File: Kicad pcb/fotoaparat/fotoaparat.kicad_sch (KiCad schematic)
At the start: 71 parts, among them IC1 Lineární Regulátor, IC3 Lineární Regulátor Displaye, J1 USB Konektor, J2 SWD, J3 LCD konektor, J4 Baterie, J5 GSD090012SEU, J6 UART, J7 Kamera, J9 Conn_01x11_Socket, U1 STM32L496RETx, U2 MCP73833-FCI/UN, Y1 8mhz krystal

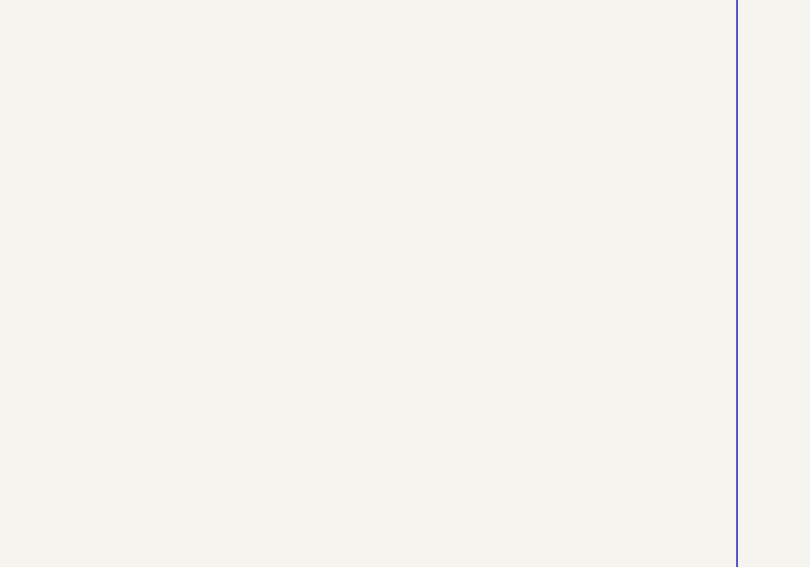
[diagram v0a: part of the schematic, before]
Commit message: Outline desky
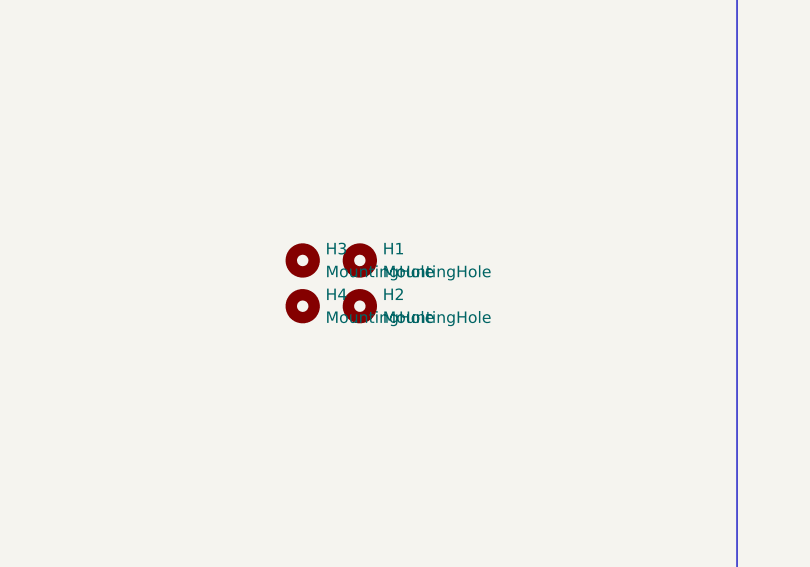
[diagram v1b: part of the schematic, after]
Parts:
- added H1, H2, H3, H4: MountingHole, MountingHole:MountingHole_3.2mm_M3, symbol Mechanical:MountingHole

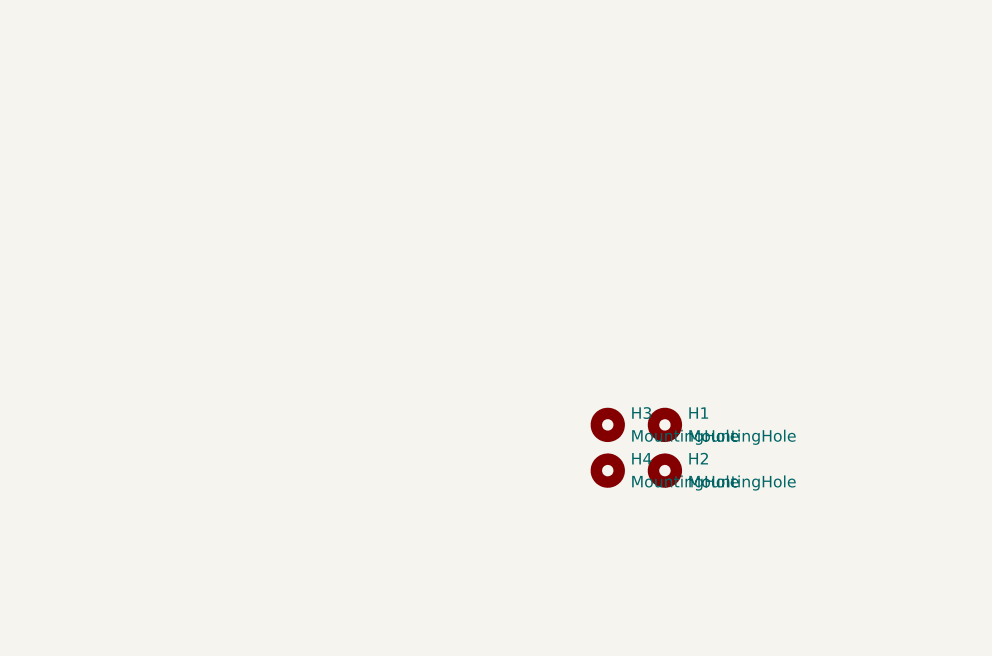
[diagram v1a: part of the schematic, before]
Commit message: První prototyp pcb
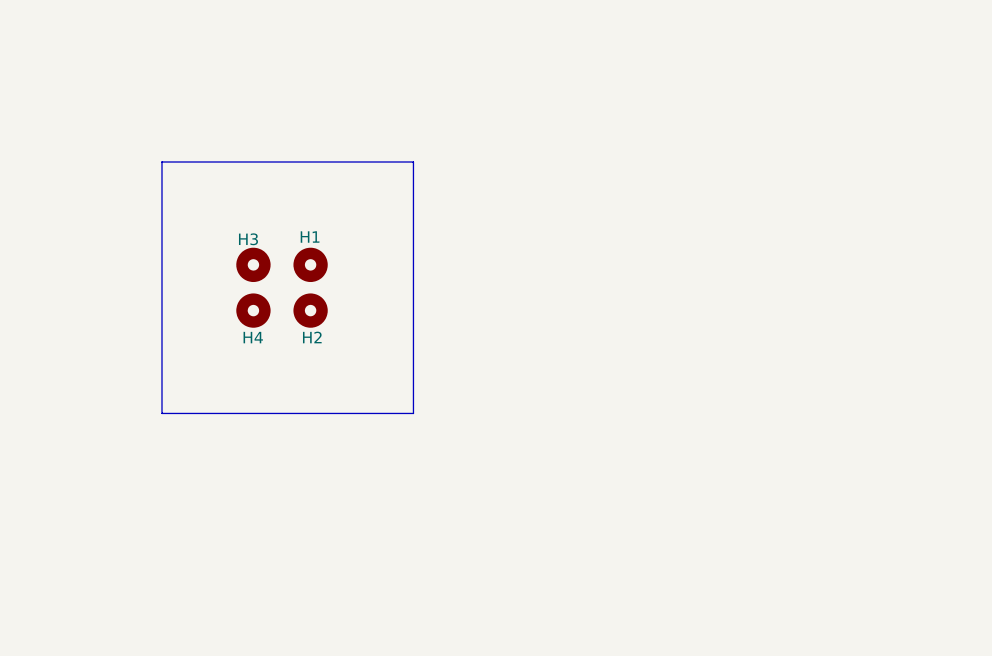
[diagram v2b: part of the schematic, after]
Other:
- moved on the sheet: H1, H2, H3, H4
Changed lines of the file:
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@@
 		(company "Vilem Maly")
 	)
+	(rectangle
+		(start -69.85 26.67)
+		(end -41.91 54.61)
+		(stroke
+			(width 0)
+			(type default)
+		)
+		(fill
+			(type none)
+		)
+	)
 	(text "Stm32 mikrokontrolér"
 		(exclude_from_sim no)
@@
 	(symbol
 		(lib_id "Mechanical:MountingHole")
-		(at -13.97 60.96 0)
+		(at -53.34 43.18 0)
 		(unit 1)
 		(exclude_from_sim no)
@@
 		(on_board yes)
 		(dnp no)
-		(fields_autoplaced yes)
 		(property "Reference" "H2"
-			(at -11.43 59.6899 0)
+			(at -54.356 46.228 0)
 			(effects
 				(font
@@
 		)
 		(property "Value" "MountingHole"
-			(at -11.43 62.2299 0)
+			(at -50.8 44.4499 0)
 			(effects
 				(font
@@
 				)
 				(justify left)
+				(hide yes)
 			)
 		)
 		(property "Footprint" "MountingHole:MountingHole_3.2mm_M3"
-			(at -13.97 60.96 0)
+			(at -53.34 43.18 0)
 			(effects
 				(font
@@
 		)
 		(property "Datasheet" "~"
-			(at -13.97 60.96 0)
+			(at -53.34 43.18 0)
 			(effects
 				(font
@@
 		)
 		(property "Description" "Mounting Hole without connection"
-			(at -13.97 60.96 0)
+			(at -53.34 43.18 0)
 			(effects
 				(font
@@
 	(symbol
 		(lib_id "Mechanical:MountingHole")
-		(at -20.32 60.96 0)
+		(at -59.69 43.18 0)
 		(unit 1)
 		(exclude_from_sim no)
@@
 		(on_board yes)
 		(dnp no)
-		(fields_autoplaced yes)
 		(property "Reference" "H4"
-			(at -17.78 59.6899 0)
+			(at -60.96 46.228 0)
 			(effects
 				(font
@@
 		)
 		(property "Value" "MountingHole"
-			(at -17.78 62.2299 0)
+			(at -57.15 44.4499 0)
 			(effects
 				(font
@@
 				)
 				(justify left)
+				(hide yes)
 			)
 		)
 		(property "Footprint" "MountingHole:MountingHole_3.2mm_M3"
-			(at -20.32 60.96 0)
+			(at -59.69 43.18 0)
 			(effects
 				(font
@@
 		)
 		(property "Datasheet" "~"
-			(at -20.32 60.96 0)
+			(at -59.69 43.18 0)
 			(effects
 				(font
@@
 		)
 		(property "Description" "Mounting Hole without connection"
-			(at -20.32 60.96 0)
+			(at -59.69 43.18 0)
 			(effects
 				(font
@@
 	(symbol
 		(lib_id "Mechanical:MountingHole")
-		(at -13.97 55.88 0)
+		(at -53.34 38.1 0)
 		(unit 1)
 		(exclude_from_sim no)
@@
 		(on_board yes)
 		(dnp no)
-		(fields_autoplaced yes)
 		(property "Reference" "H1"
-			(at -11.43 54.6099 0)
+			(at -54.61 35.052 0)
 			(effects
 				(font
@@
 		)
 		(property "Value" "MountingHole"
-			(at -11.43 57.1499 0)
+			(at -50.8 39.3699 0)
 			(effects
 				(font
@@
 				)
 				(justify left)
+				(hide yes)
 			)
 		)
 		(property "Footprint" "MountingHole:MountingHole_3.2mm_M3"
-			(at -13.97 55.88 0)
+			(at -53.34 38.1 0)
 			(effects
 				(font
@@
 		)
 		(property "Datasheet" "~"
-			(at -13.97 55.88 0)
+			(at -53.34 38.1 0)
 			(effects
 				(font
@@
 		)
 		(property "Description" "Mounting Hole without connection"
-			(at -13.97 55.88 0)
+			(at -53.34 38.1 0)
 			(effects
 				(font
@@
 	(symbol
 		(lib_id "Mechanical:MountingHole")
-		(at -20.32 55.88 0)
+		(at -59.69 38.1 0)
 		(unit 1)
 		(exclude_from_sim no)
@@
 		(on_board yes)
 		(dnp no)
-		(fields_autoplaced yes)
 		(property "Reference" "H3"
-			(at -17.78 54.6099 0)
+			(at -61.468 35.306 0)
 			(effects
 				(font
@@
 		)
 		(property "Value" "MountingHole"
-			(at -17.78 57.1499 0)
+			(at -74.168 38.354 0)
 			(effects
 				(font
@@
 				)
 				(justify left)
+				(hide yes)
 			)
 		)
 		(property "Footprint" "MountingHole:MountingHole_3.2mm_M3"
-			(at -20.32 55.88 0)
+			(at -59.69 38.1 0)
 			(effects
 				(font
@@
 		)
 		(property "Datasheet" "~"
-			(at -20.32 55.88 0)
+			(at -59.69 38.1 0)
 			(effects
 				(font
@@
 		)
 		(property "Description" "Mounting Hole without connection"
-			(at -20.32 55.88 0)
+			(at -59.69 38.1 0)
 			(effects
 				(font
